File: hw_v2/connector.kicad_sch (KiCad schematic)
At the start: 22 parts, among them J1 Conn_02x24_Counter_Clockwise, J14 Conn_01x04, U11 L78M05ABDT-TR, U19 L78M05ABDT-TR, U25 74LVC2G17, U26 74LVC2G17, U8 AMS1117-3.3

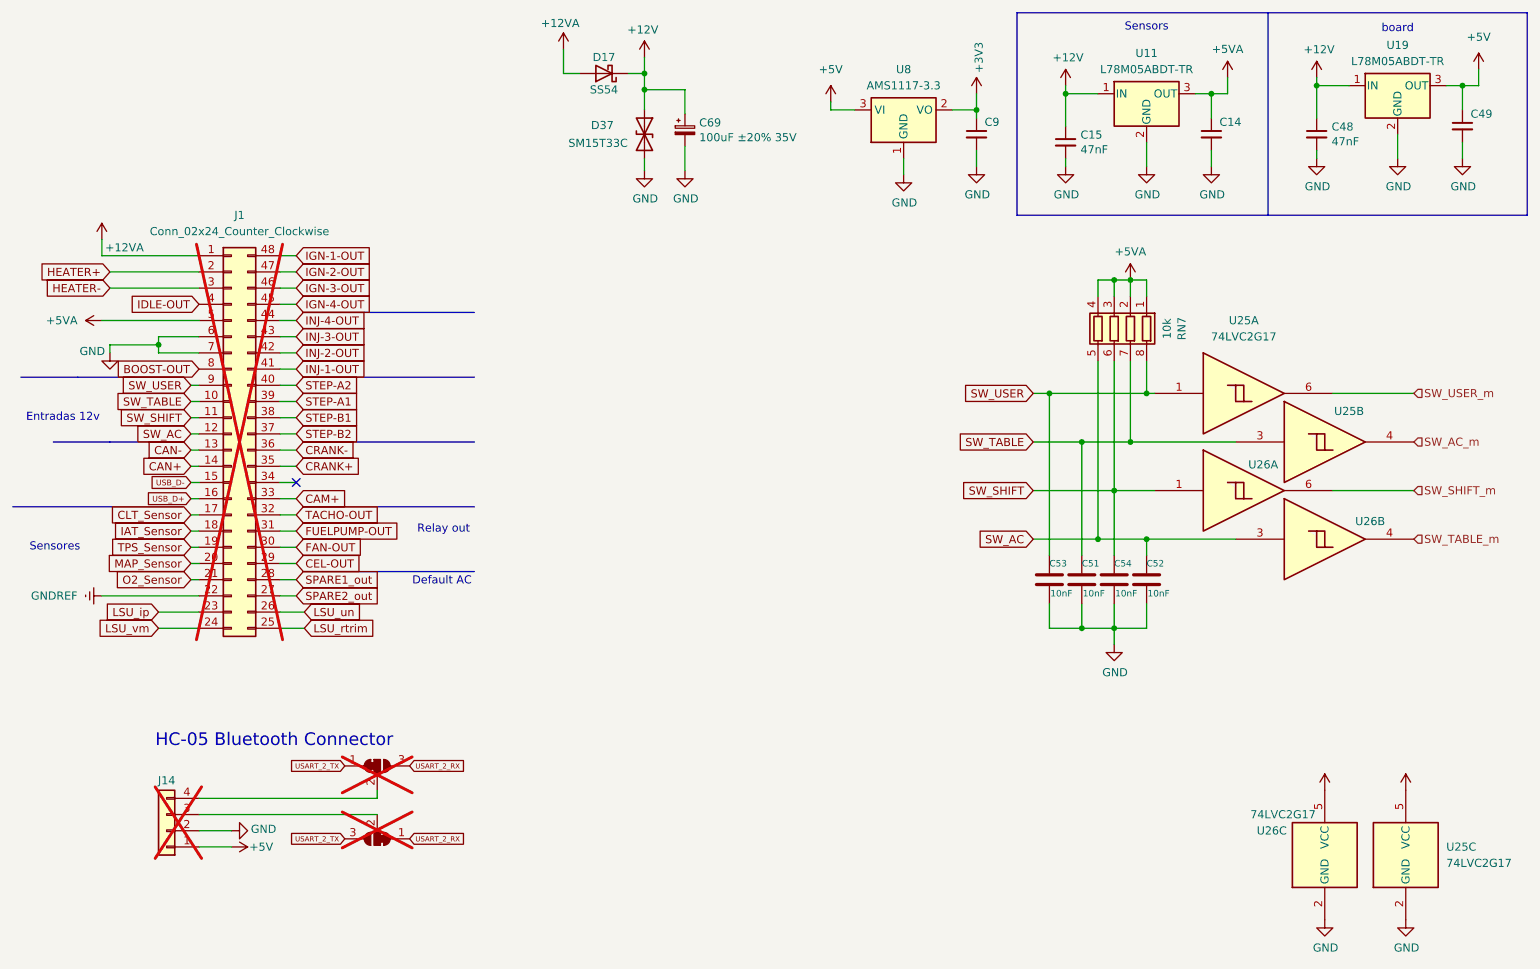
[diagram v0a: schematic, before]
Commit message: planito mas catolico
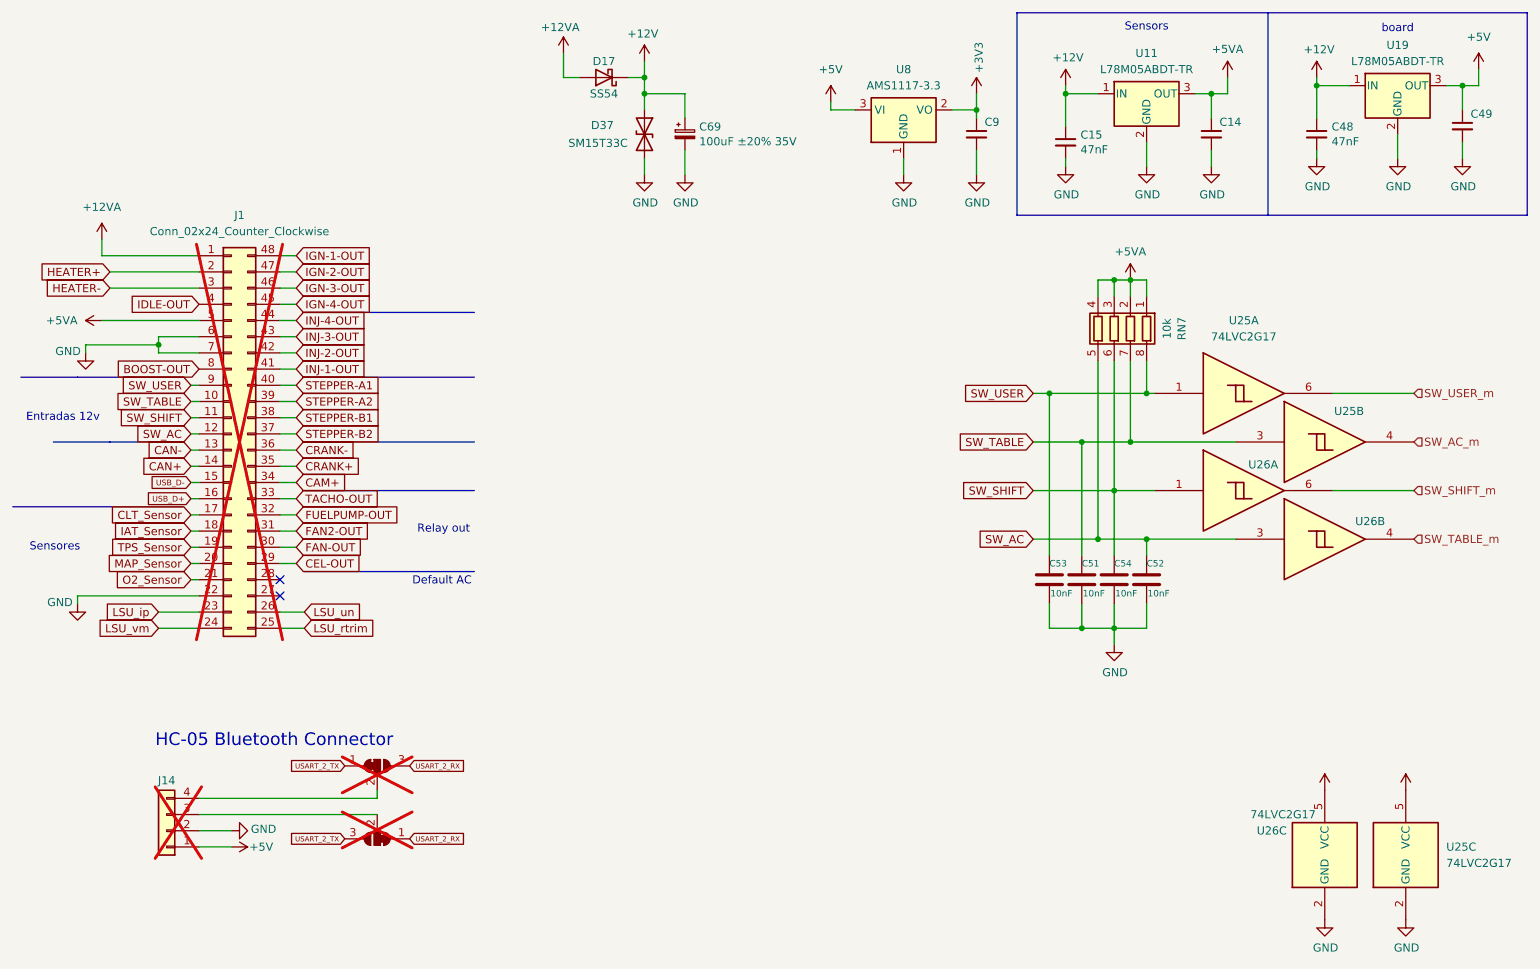
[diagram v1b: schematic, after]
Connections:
- net GNDREF is gone; now on net GND: J1.22 (Pin_22)
- net CAM+: now also J1.34 (Pin_34); no longer J1.33 (Pin_33)
- net FUELPUMP-OUT: now also J1.32 (Pin_32); no longer J1.31 (Pin_31)
- net TACHO-OUT: now also J1.33 (Pin_33); no longer J1.32 (Pin_32)
- net SPARE1_out: no longer names the net of J1.28 (Pin_28)
- net SPARE2_out: no longer names the net of J1.27 (Pin_27)
- net STEP-A1 renamed STEPPER-A2
- net STEP-A2 renamed STEPPER-A1
- net STEP-B1 renamed STEPPER-B1
- net STEP-B2 renamed STEPPER-B2
- new net FAN2-OUT: J1.31 (Pin_31)
- no-connect marks 1 -> 2
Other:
- moved on the sheet: C69, D17
